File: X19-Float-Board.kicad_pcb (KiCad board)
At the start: 2 copper layers, 86 x 86 mm, 41 parts, among them J1 USB4220-03-1040-C_REVA, SW2 SW_Nidec_CAS-120A1, U2 STM32C542CCT6, U3 STM32G431RBT6, U4 INA228AIDGSR, U5 TPS561208DDCR, U6 TMP1075NDRLR

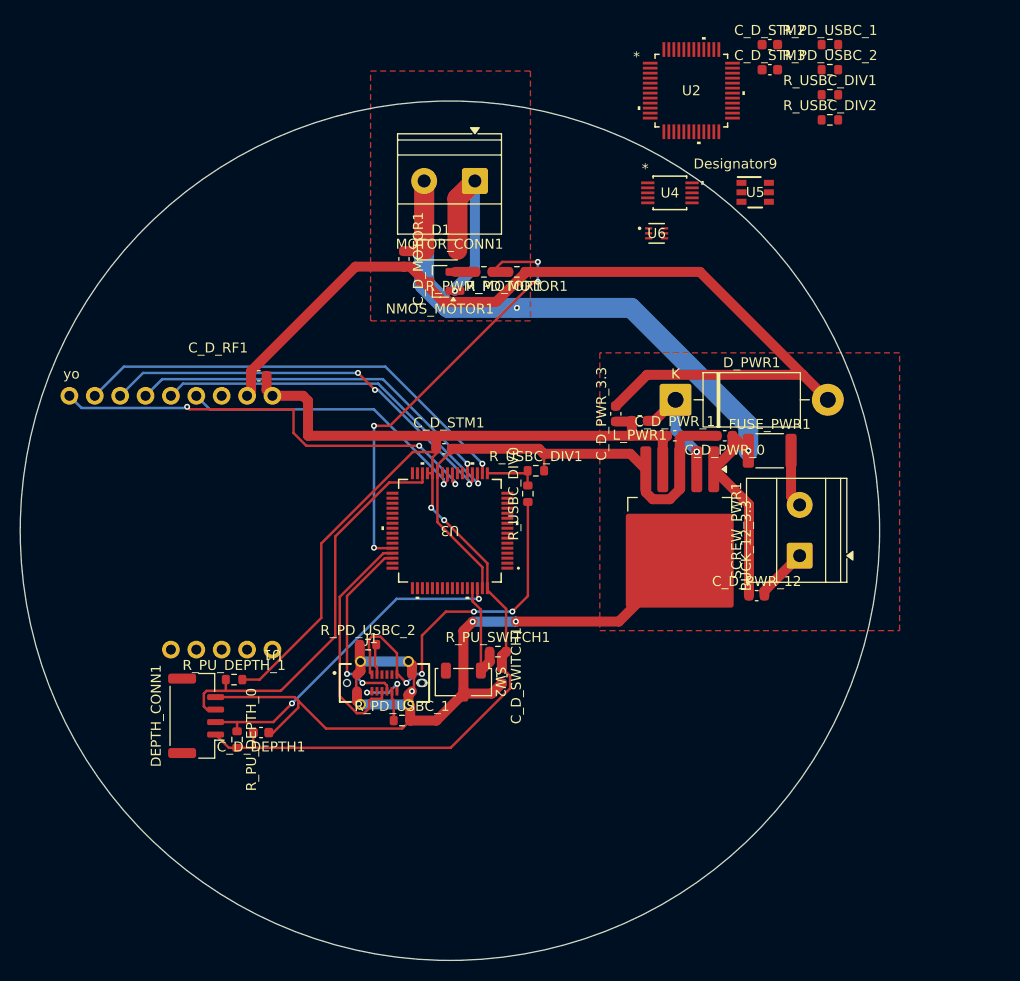
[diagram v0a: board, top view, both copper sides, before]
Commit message: footprints
footprints
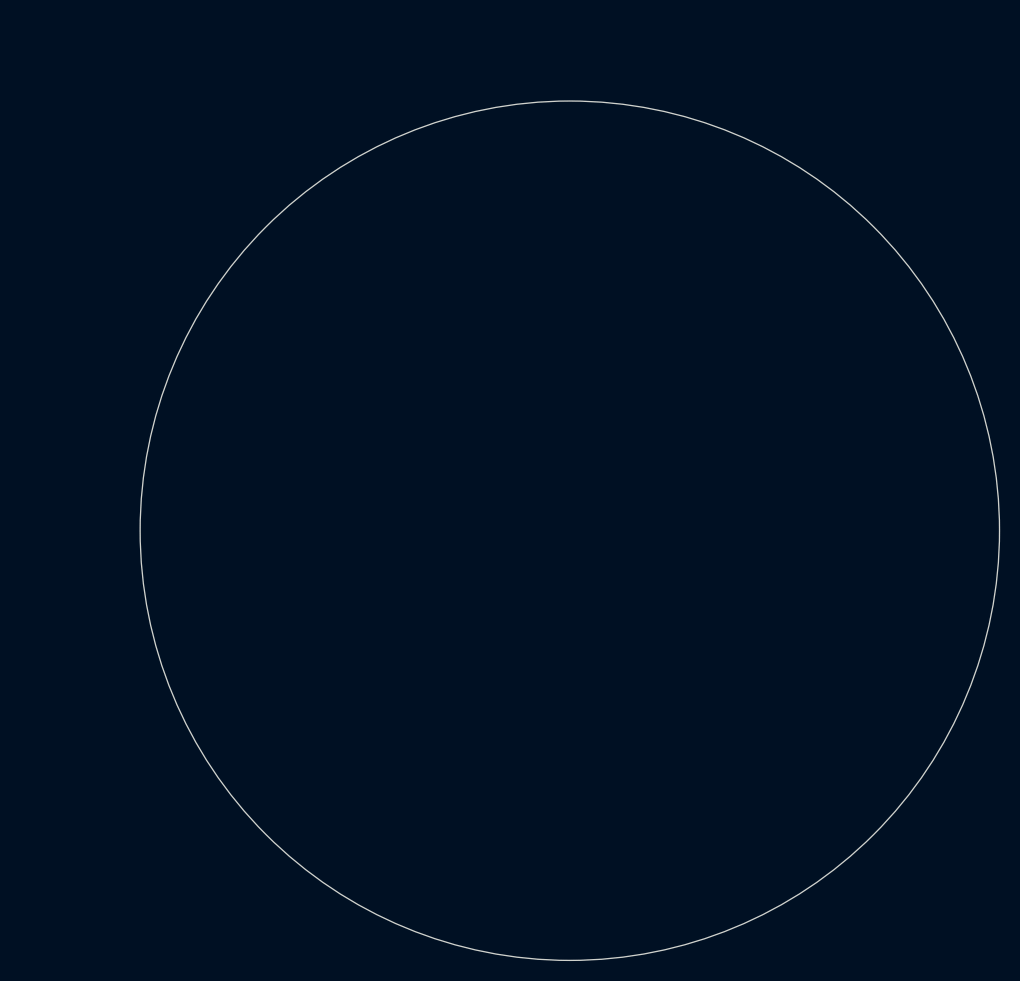
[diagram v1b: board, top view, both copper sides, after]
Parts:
- removed BUCK_12_3.3: LM2596S-3.3, Package_TO_SOT_SMD:TO-263-5_TabPin3
- removed C_D_DEPTH1, C_D_MOTOR1, C_D_RF1, C_D_STM1, C_D_STM2, C_D_STM3, C_D_SWITCH1: 100nF, Capacitor_SMD:C_0603_1608Metric
- removed C_D_PWR_0: 680µF, Capacitor_SMD:C_0603_1608Metric
- removed C_D_PWR_1: 220µF, Capacitor_SMD:C_0603_1608Metric
- removed C_D_PWR_12, C_D_PWR_3.3: 4.7µF, Capacitor_SMD:C_0603_1608Metric
- removed D1: D_MOTOR, Diode_SMD:D_SOD-123
- removed DEPTH_CONN1: Conn_01x04_Pin, Connector_JST:JST_GH_BM04B-GHS-TBT_1x04-1MP_P1.25mm_Vertical
- removed D_PWR1: 1N5822, Diode_THT:D_DO-201AD_P15.24mm_Horizontal
- removed FUSE_PWR1: 2A 12V PTC fuse, Fuse:Fuse_1812_4532Metric
- removed J1: USB4220-03-1040-C_REVA, usbc:GCT_USB4220-03-1040-C_REVA
- removed L_PWR1: 33µH, Inductor_SMD:L_0603_1608Metric
- removed MOTOR_CONN1: Motor, TerminalBlock_Phoenix:TerminalBlock_Phoenix_MKDS-1,5-2-5.08_1x02_P5.08mm_Horizontal
- removed NMOS_MOTOR1: NMOS, Package_TO_SOT_SMD:SOT-23_Handsoldering
- removed R_PD_MOTOR1, R_PU_SWITCH1: 10kΩ, Resistor_SMD:R_0603_1608Metric
- removed R_PD_USBC_1 (x2): 5.1k, Resistor_SMD:R_0603_1608Metric
- removed R_PD_USBC_2 (x2): 5.1kΩ, Resistor_SMD:R_0603_1608Metric
- removed R_PU_DEPTH_0, R_PU_DEPTH_1: 4.7kΩ, Resistor_SMD:R_0603_1608Metric
- removed R_PWM_MOTOR1: 220Ω, Resistor_SMD:R_0603_1608Metric
- removed R_USBC_DIV0, R_USBC_DIV1: 20kΩ, Resistor_SMD:R_0603_1608Metric
- removed R_USBC_DIV1, R_USBC_DIV2: 10kΩ, Resistor_SMD:R_0603_1608Metric
- removed SCREW_PWR1: Screw_Terminal_01x02, TerminalBlock_Phoenix:TerminalBlock_Phoenix_MKDS-1,5-2-5.08_1x02_P5.08mm_Horizontal
- removed SW2: SW_Nidec_CAS-120A1, Button_Switch_SMD:Nidec_Copal_CAS-120A
- removed U1: ~, customrf:rf module
- removed U2: STM32C542CCT6, rov_logic:LQFP48-7X7
- removed U3: STM32G431RBT6, stm32:LQFP64-10x10mm
- removed U4: INA228AIDGSR, CustomFootprints:VSSOP10_DGS_TEX
- removed U5: TPS561208DDCR, CustomFootprints:DDC0006A_N
- removed U6: TMP1075NDRLR, CustomFootprints:SOT5X3-6_DRL_TEX
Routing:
- net GND: track 241.5 -> 0.00 mm, vias 6 -> 0
- net 3.3 V: track 149.3 -> 0.00 mm, vias 3 -> 0
- net 12 V: track 80.6 -> 0.00 mm, vias 2 -> 0
- net /rf/RF RST: track 45.4 -> 0.00 mm, vias 3 -> 0
- net /Motor/Motor PWM: track 45.1 -> 0.00 mm, vias 4 -> 0
- net /rf/RF NSS: track 45.0 -> 0.00 mm, vias 1 -> 0
- net /rf/RF MOSI: track 41.9 -> 0.00 mm, vias 3 -> 0
- net /sensor/Depth SDA: track 41.1 -> 0.00 mm
- net VBUS_A: track 38.1 -> 0.00 mm, vias 4 -> 0
- net /rf/RF MISO: track 37.4 -> 0.00 mm, vias 1 -> 0
- net /rf/RF SCK: track 36.4 -> 0.00 mm, vias 1 -> 0
- net /sensor/Depth SCL: track 33.5 -> 0.00 mm, vias 2 -> 0
- net /rf/RF INT: track 30.0 -> 0.00 mm, vias 1 -> 0
- net Net-(J1-DN2): track 23.7 -> 0.00 mm
- net Net-(D1-A): track 19.5 -> 0.00 mm, vias 1 -> 0
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- removed copper zone on F.Cu, net 12 V
- removed copper zone on F.Cu, net GND
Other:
- board text removed: "yo"
